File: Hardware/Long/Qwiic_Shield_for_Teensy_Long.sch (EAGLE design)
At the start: 21 parts, among them J1 QWIIC_RA, J2 QWIIC_RA, J4 QWIIC_Vertical, J5 ALT PWR

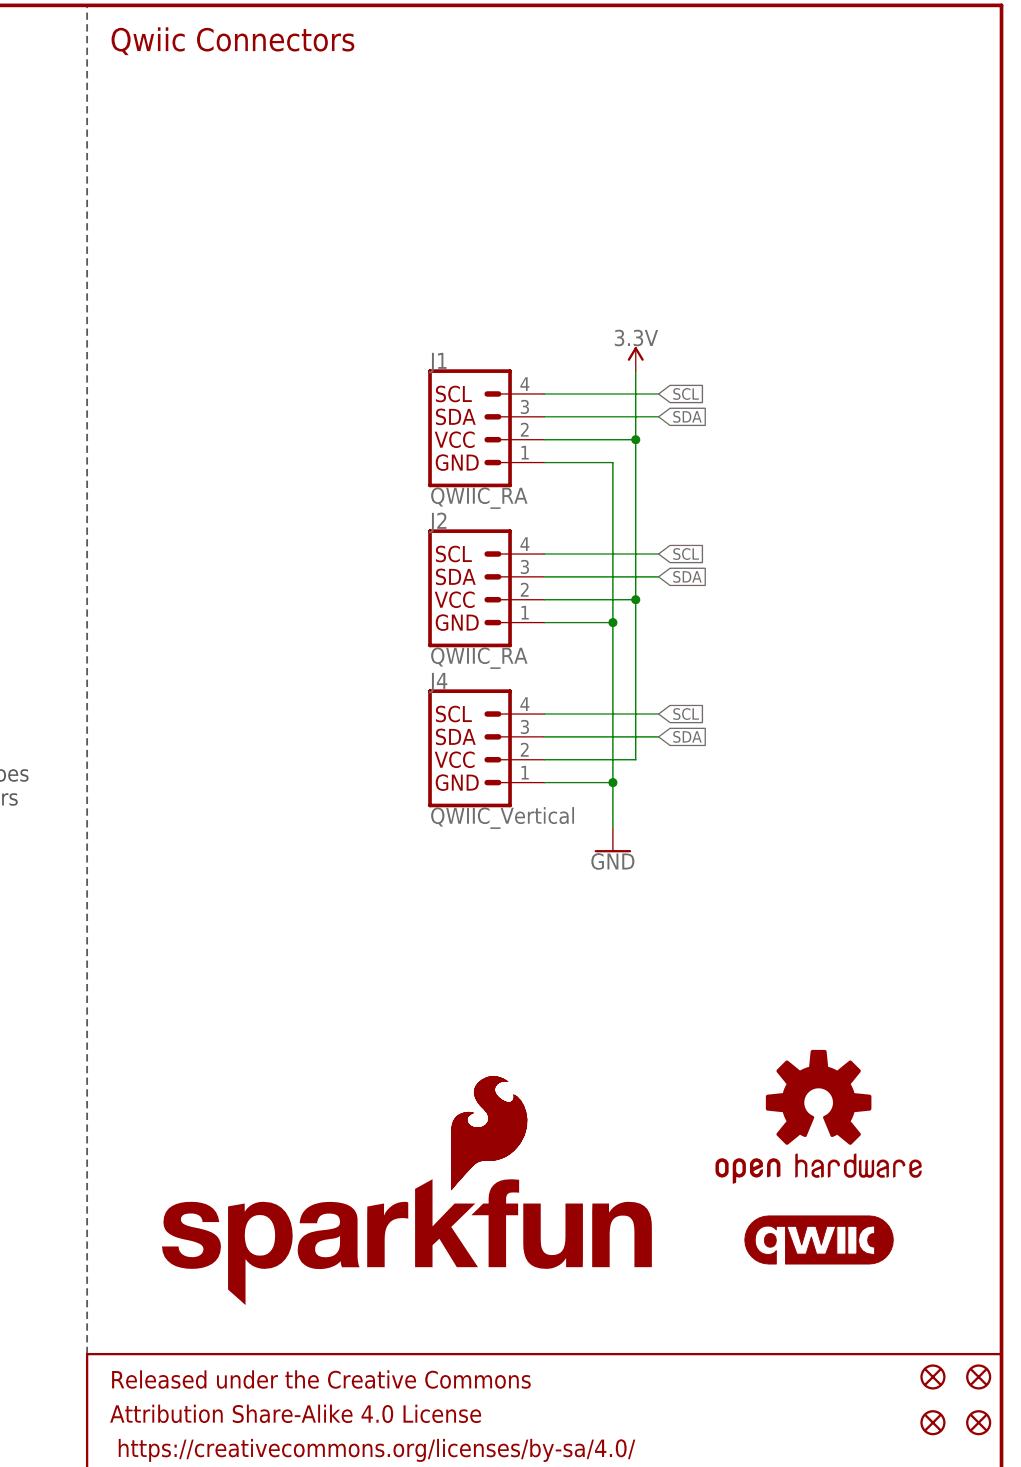
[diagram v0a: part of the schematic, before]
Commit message: Long version routed
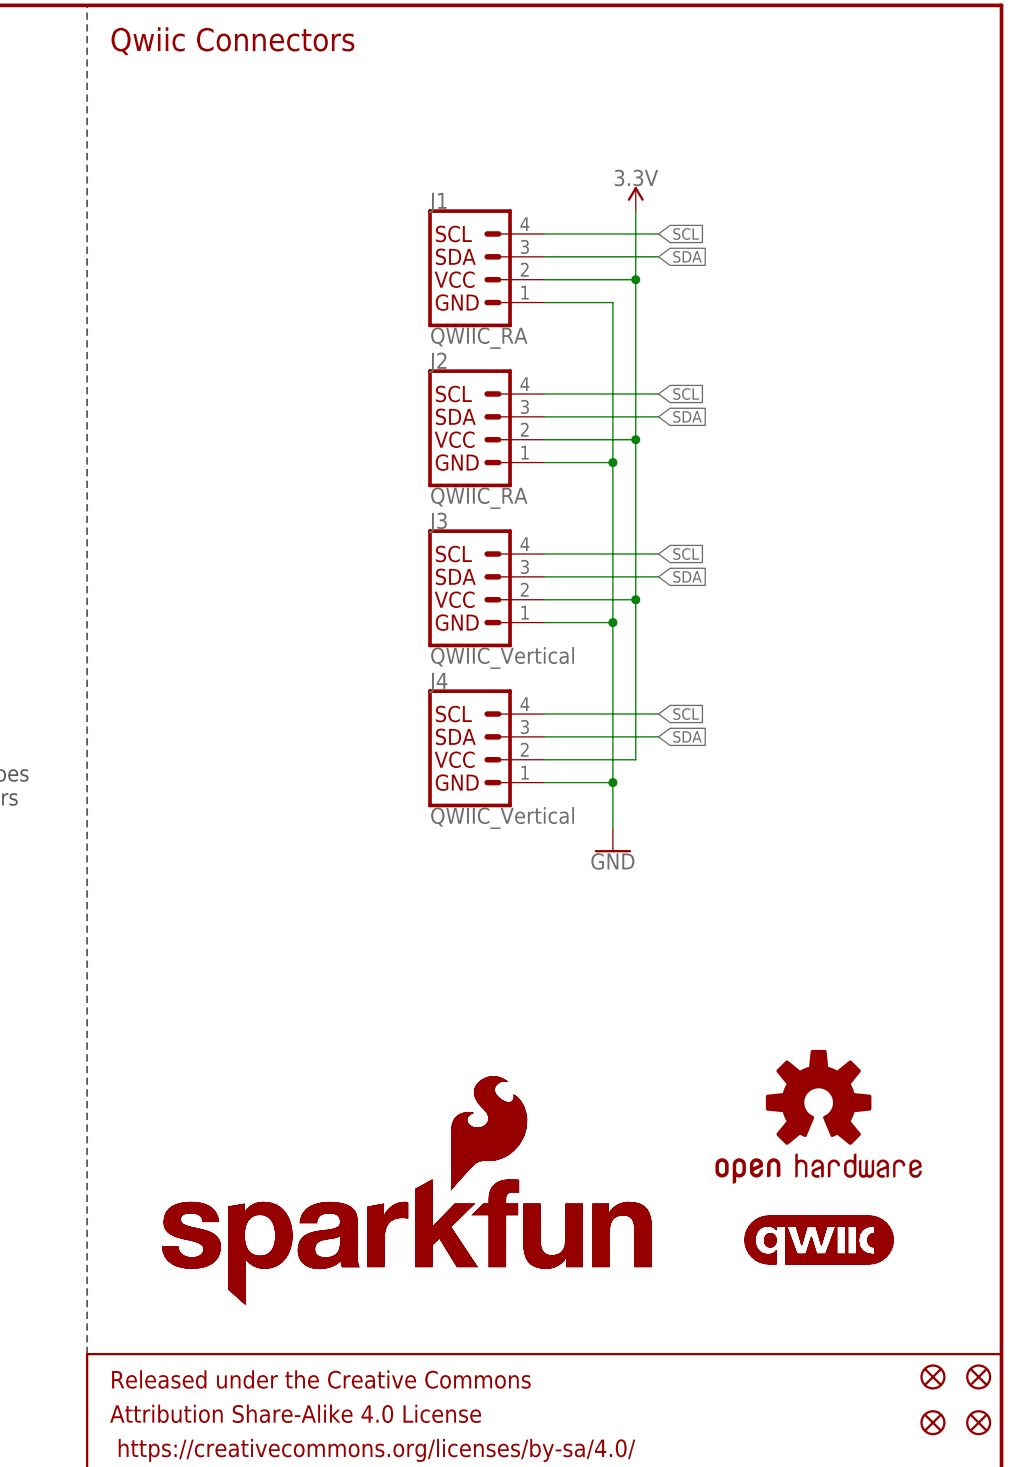
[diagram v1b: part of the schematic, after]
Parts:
- added J3: QWIIC_Vertical, SparkFun-Connectors:QWIIC_CONNECTOR
- added LOGO5: QWIIC_LOGO_5MM, SparkFun-Aesthetics:QWIIC_LOGO_5MM
- LOGO2: value SFE_LOGO_FLAME.1_INCH -> SFE_LOGO_NAME_FLAME.1_INCH; device SparkFun-Aesthetics:SFE_LOGO_FLAME.1_INCH -> SparkFun-Aesthetics:SFE_LOGO_NAME_FLAME.1_INCH
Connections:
- net 3.3V: now also J3.2
- net GND: now also J3.1
- net SCL: now also J3.4
- net SDA: now also J3.3
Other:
- moved on the sheet: J1, J2
